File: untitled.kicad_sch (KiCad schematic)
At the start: 27 parts, among them M2 M2 front right, M3 M3 rear right, M4 m4 rear left, U10 AON7410, U11 UCC27511ADBV, U12 AON7410, U7 UCC27511ADBV, U8 AON7410, U9 UCC27511ADBV

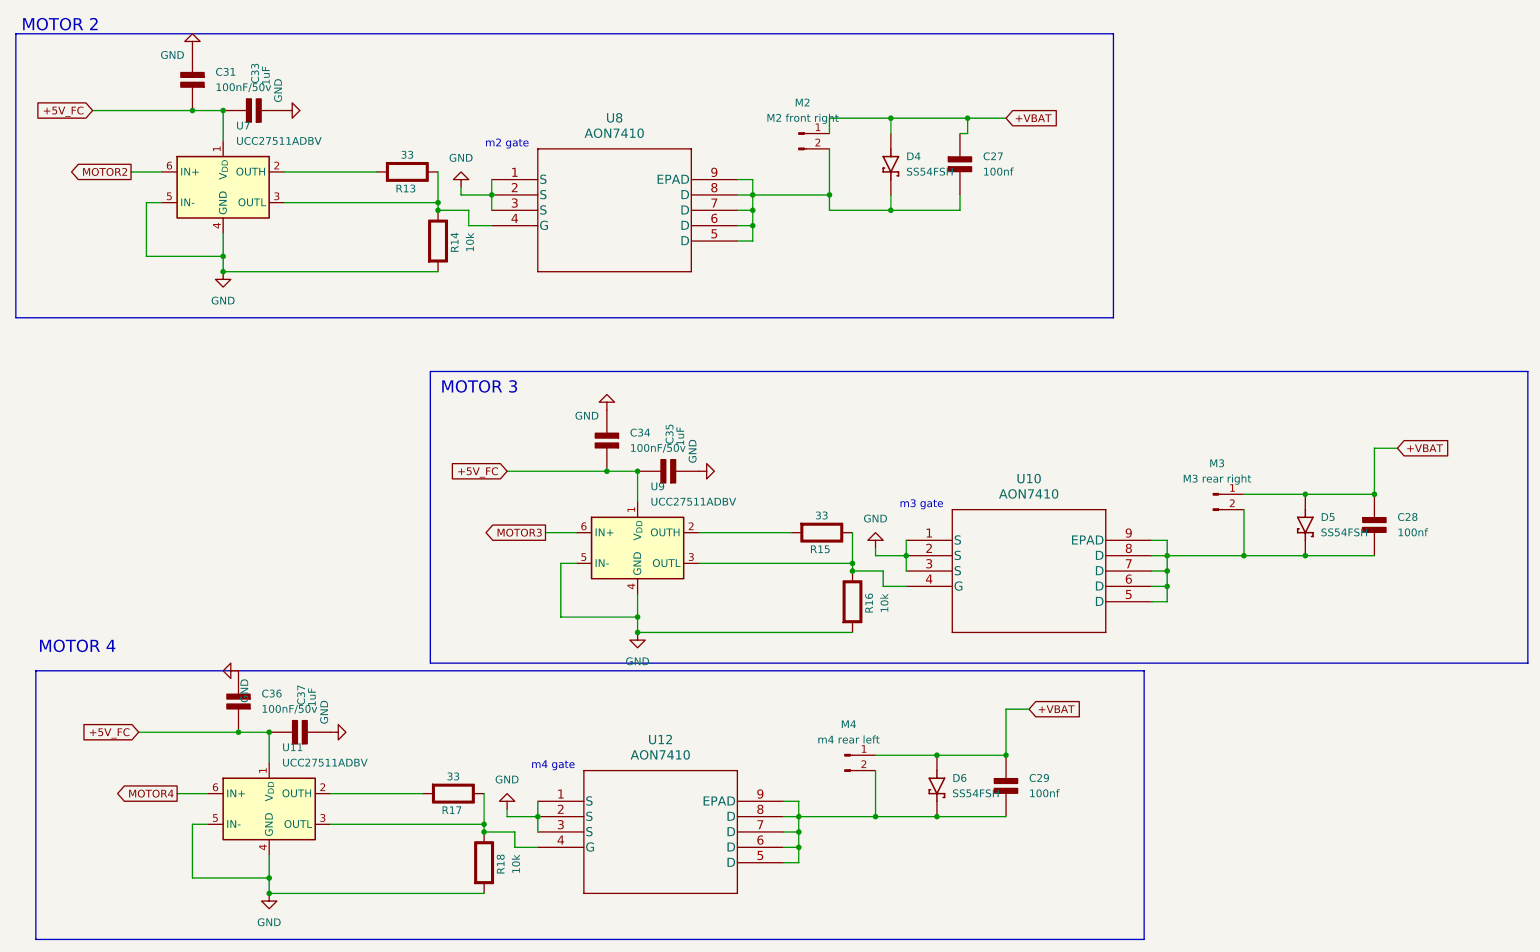
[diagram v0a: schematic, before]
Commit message: update
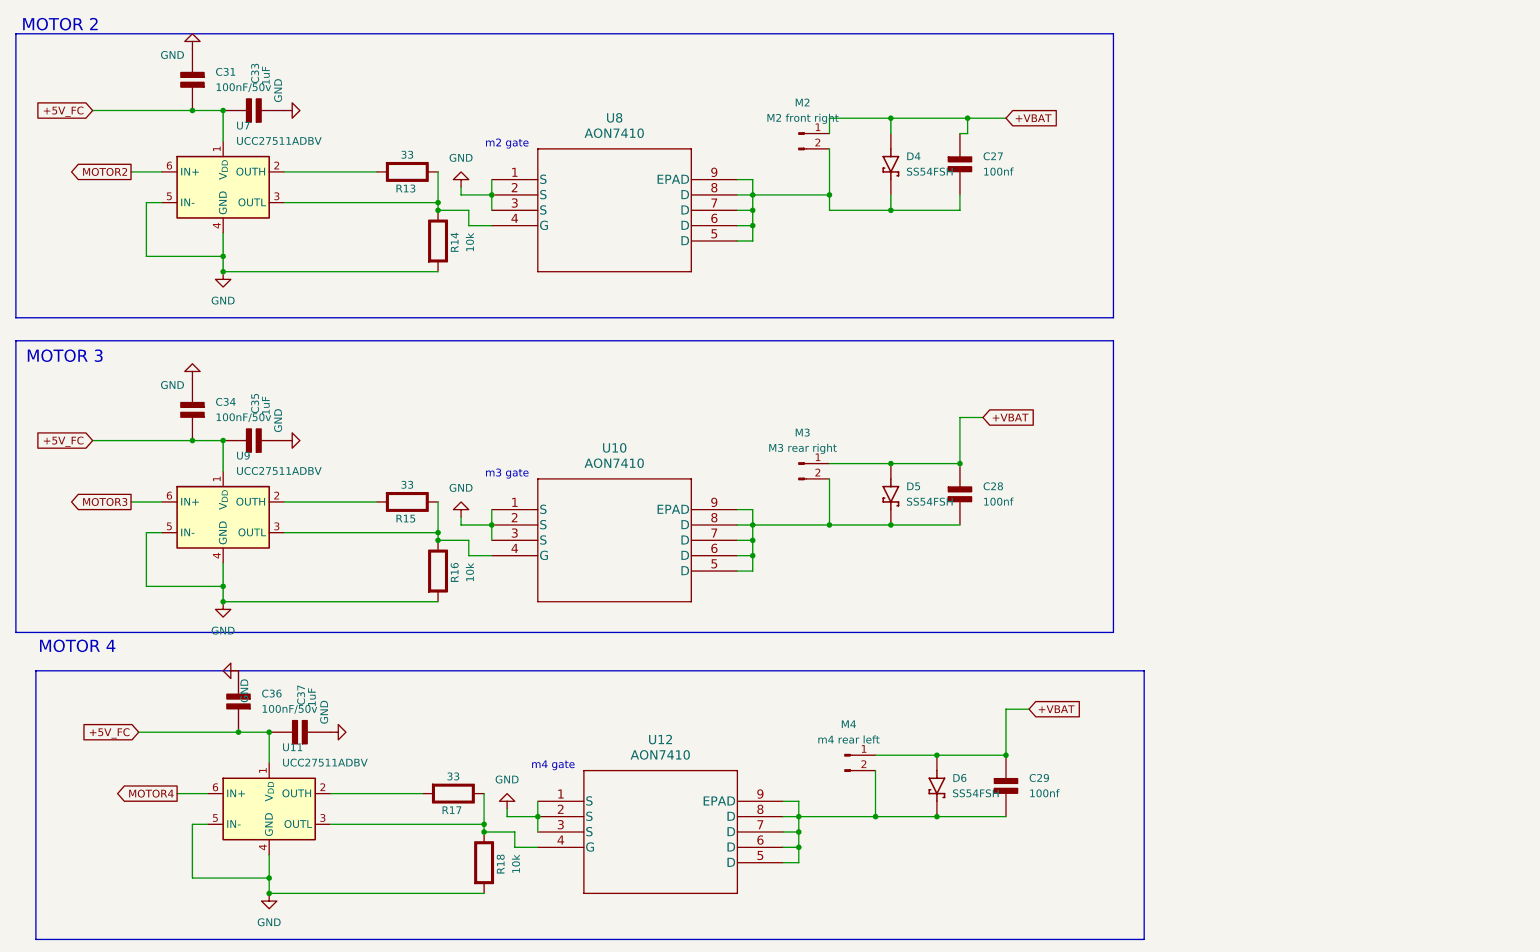
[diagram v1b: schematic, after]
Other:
- moved on the sheet: C28, C34, C35, D5, M3, R15, R16, U10, U9
